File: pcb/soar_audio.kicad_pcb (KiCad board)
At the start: 4 copper layers, 103 parts, among them J1 RJ45-FLAPS, J2 RJ12-FLAPS, J3 HEADER_4, J4 Screw_Terminal_01x02, J5 RJ45-CAN, J6 HEADER_4, J7 HEADER_2, Q1 AO3401A, U1 LV2842X, U3 SN65HVD231, U4 PAM8302AAS, U6 BP

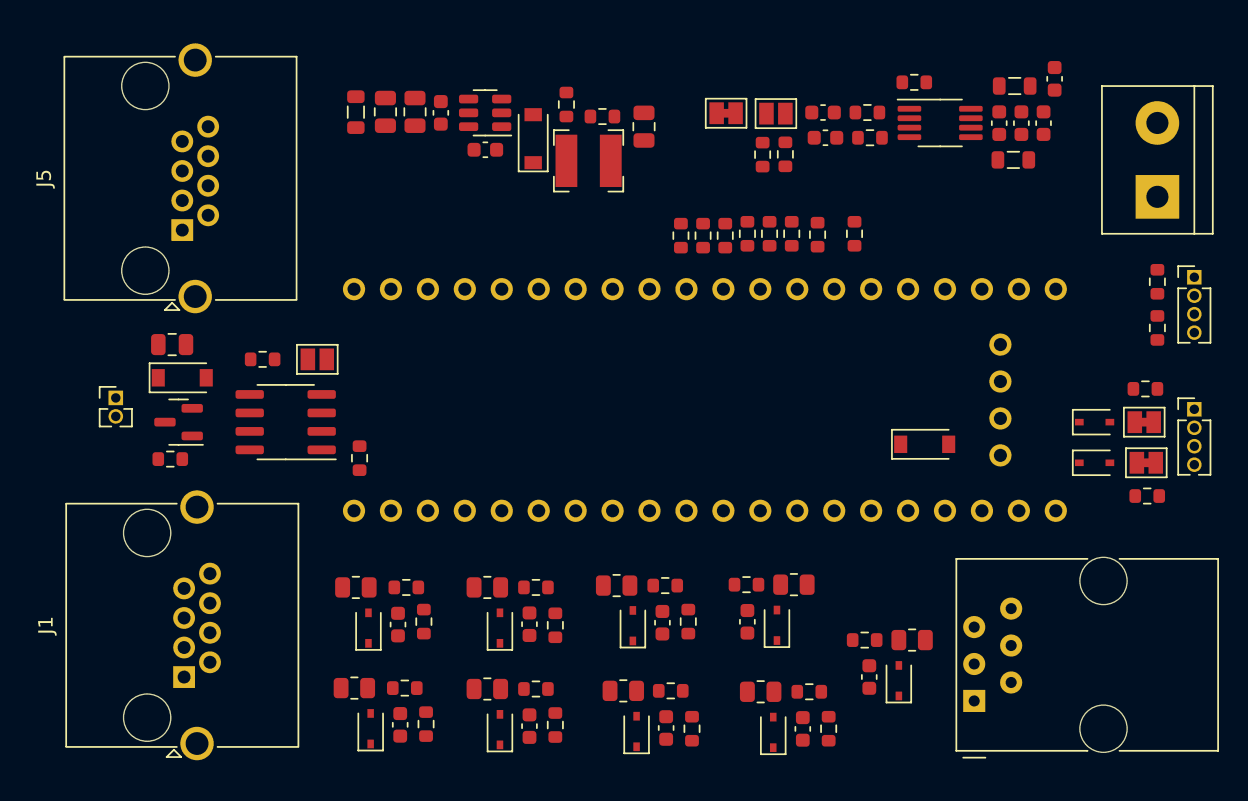
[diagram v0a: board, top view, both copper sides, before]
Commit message: some more steps done
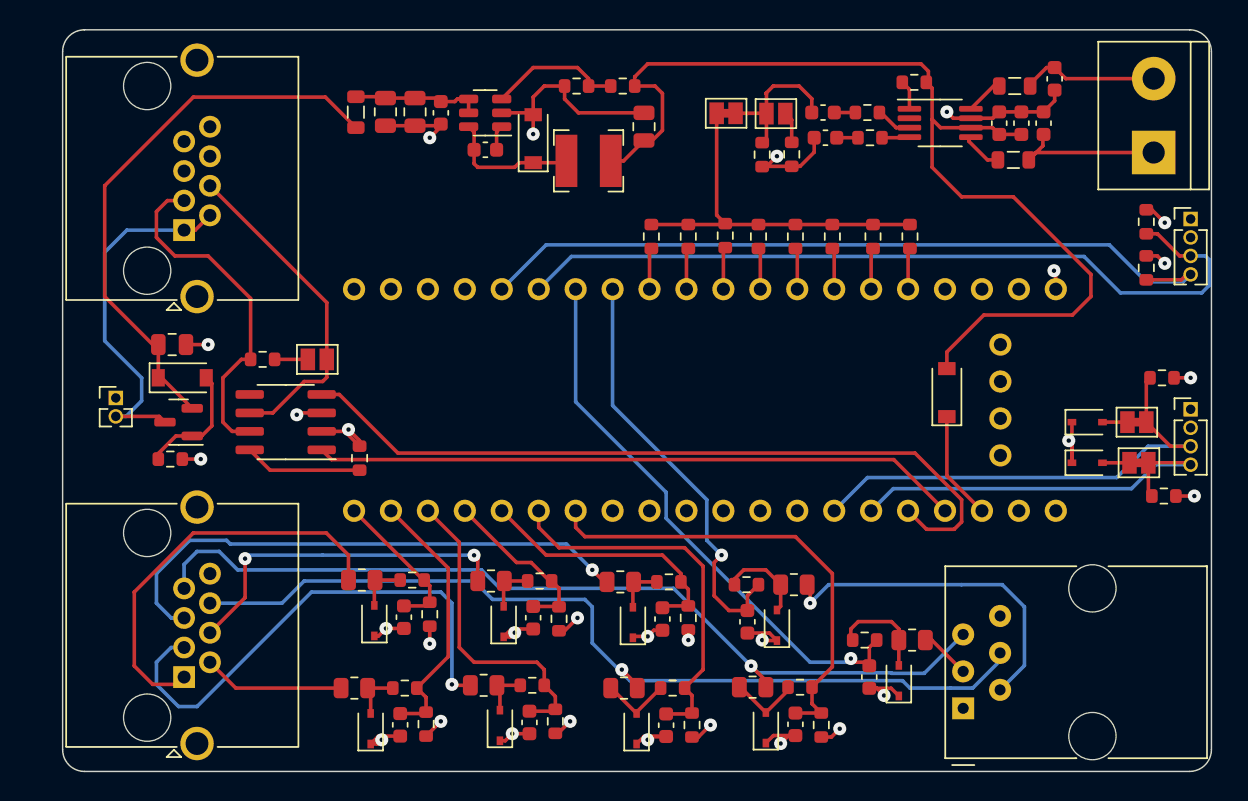
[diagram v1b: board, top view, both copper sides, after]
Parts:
- moved R28 11.7 mm to (144.5, 107.4)
- moved D15 11.7 mm to (140.7, 107.8)
- moved R26 11.7 mm to (139.9, 105.0)
- moved R27 11.7 mm to (143.2, 105.0)
- moved C20 11.7 mm to (142.7, 107.5)
- moved D12 11.4 mm to (131.6, 114.8)
- moved R17 11.4 mm to (130.5, 112.1)
- moved R18 11.4 mm to (133.8, 112.1)
- moved R19 11.4 mm to (135.4, 114.6)
- moved C17 11.4 mm to (133.6, 114.6)
- moved C21 9.40 mm to (143.0, 114.8)
- moved D16 9.40 mm to (141.0, 115.1)
- moved R29 9.40 mm to (140.1, 112.3)
- moved R30 9.40 mm to (143.4, 112.3)
- moved R31 9.40 mm to (144.8, 114.8)
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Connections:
- U6 pad VBAT: unconnected-(U6-PadVBAT) -> +3V3
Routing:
- net GND: track 0.00 -> 72.7 mm, vias 0 -> 17
- net +5V: track 0.00 -> 72.0 mm
- net Flaps_Input6: track 0.00 -> 62.5 mm, vias 0 -> 1
- net Flaps_Input7: track 0.00 -> 62.1 mm, vias 0 -> 1
- net SCL2: track 0.00 -> 55.1 mm
- net SDA2: track 0.00 -> 53.1 mm
- net CAN_RX: track 0.00 -> 52.9 mm
- net CAN_TX: track 0.00 -> 44.6 mm
- net VSUPPLY: track 0.00 -> 38.8 mm
- net ADC_In2: track 0.00 -> 38.5 mm, vias 0 -> 1
- net Flaps_Input5: track 0.00 -> 37.5 mm, vias 0 -> 1
- net Flaps_Input3: track 0.00 -> 35.3 mm, vias 0 -> 1
- net SCL: track 0.00 -> 33.2 mm
- net Flaps_In7: track 0.00 -> 32.3 mm
- net ADC_In1: track 0.00 -> 29.2 mm, vias 0 -> 1
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- added copper zone on In2.Cu, net +3V3
- added copper zone on In1.Cu, net GND
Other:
- board outline added: 79 x 51 mm
